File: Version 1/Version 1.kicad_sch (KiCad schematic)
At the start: 85 parts, among them J1 Conn_01x05, Q1 IPP015N04NF2SAKMA1, Q2 IPP015N04NF2SAKMA1, Q3 IPP015N04NF2SAKMA1, Q4 IPP015N04NF2SAKMA1, Q5 IPP015N04NF2SAKMA1, Q6 IPP015N04NF2SAKMA1, U1 TPS62932, U2 TPS62932, U3 TPS62932, U4 IRS2004, U5 IRS2004, U6 IRS2004, U7 YAAJ_BlackPill_SWD_BreakoutV2, U8 ACS712xLCTR-05B

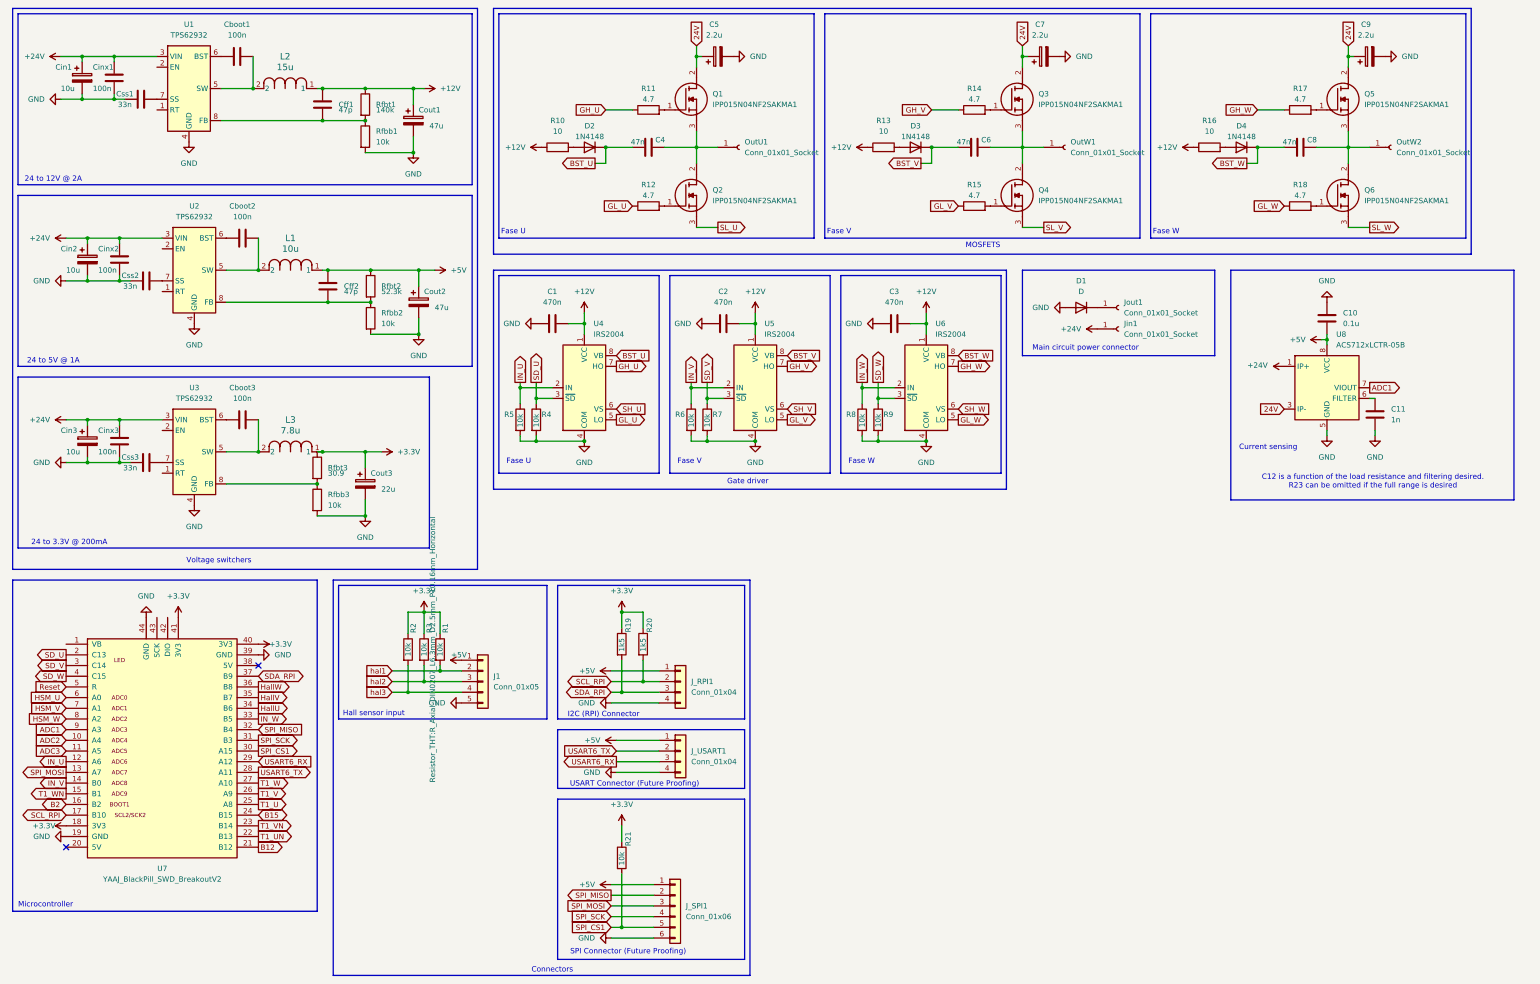
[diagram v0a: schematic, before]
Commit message: updated
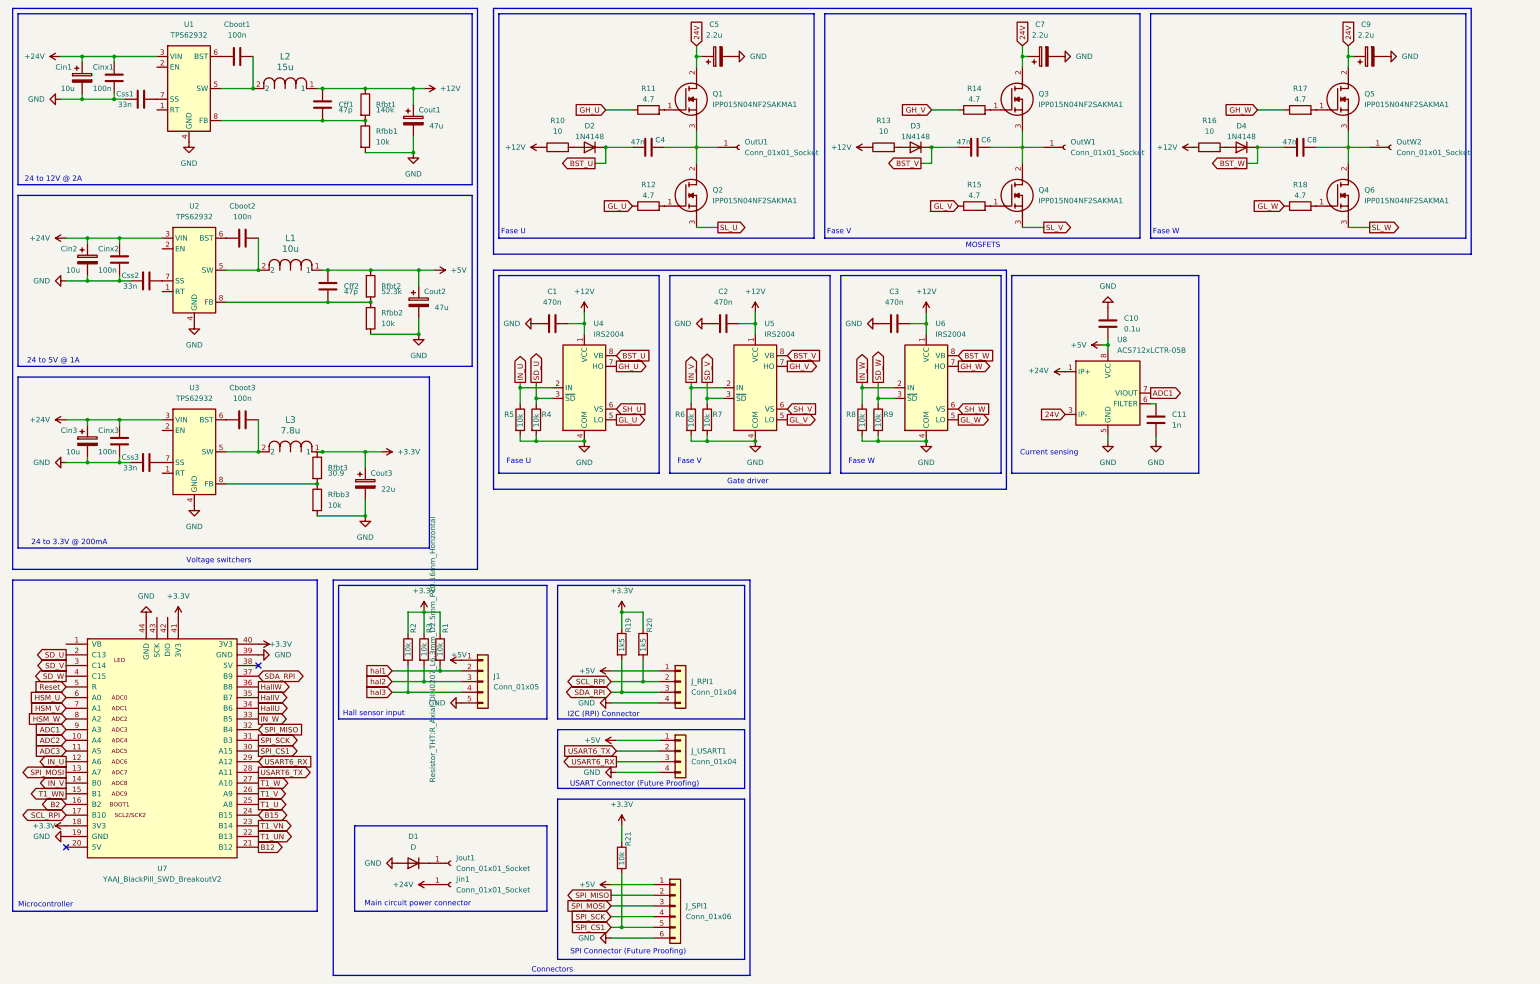
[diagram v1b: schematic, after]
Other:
- note removed: "C12 is a function of the load resistance and filtering desired. R23 can be omitted if the full range is desired"
- moved on the sheet: C10, C11, D1, Jin1, Jout1, U8
